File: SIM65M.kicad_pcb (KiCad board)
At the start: 4 copper layers, 40 x 40 mm, 25 parts, among them J1 Conn_01x11_Pin, J2 U.FL-R-SMT_10_, Q1 AO3400A, Q2 DTC143ZUAT106, Q3 DTC143ZUAT106, U1 SIM65M_C7495025, U2 BWGNSCNX25-25W4, U5 XC6206P282MR-G

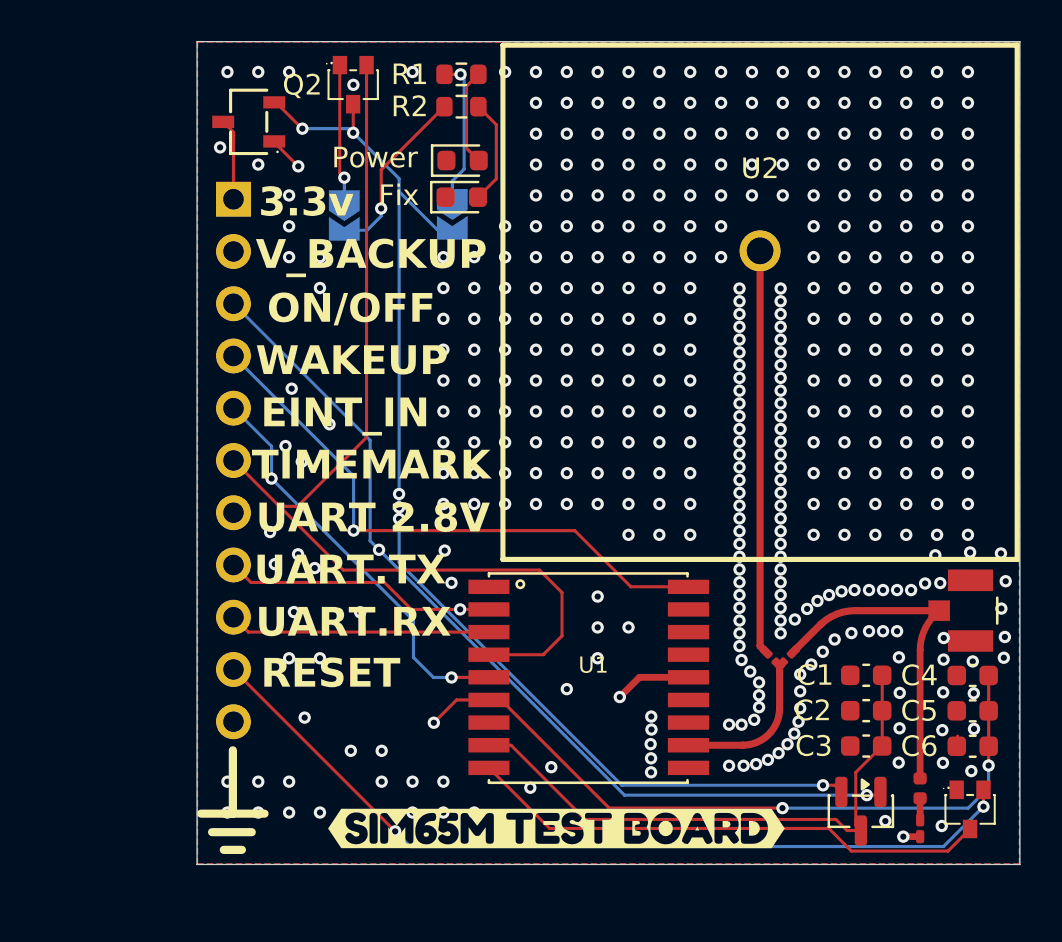
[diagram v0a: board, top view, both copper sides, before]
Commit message: carga
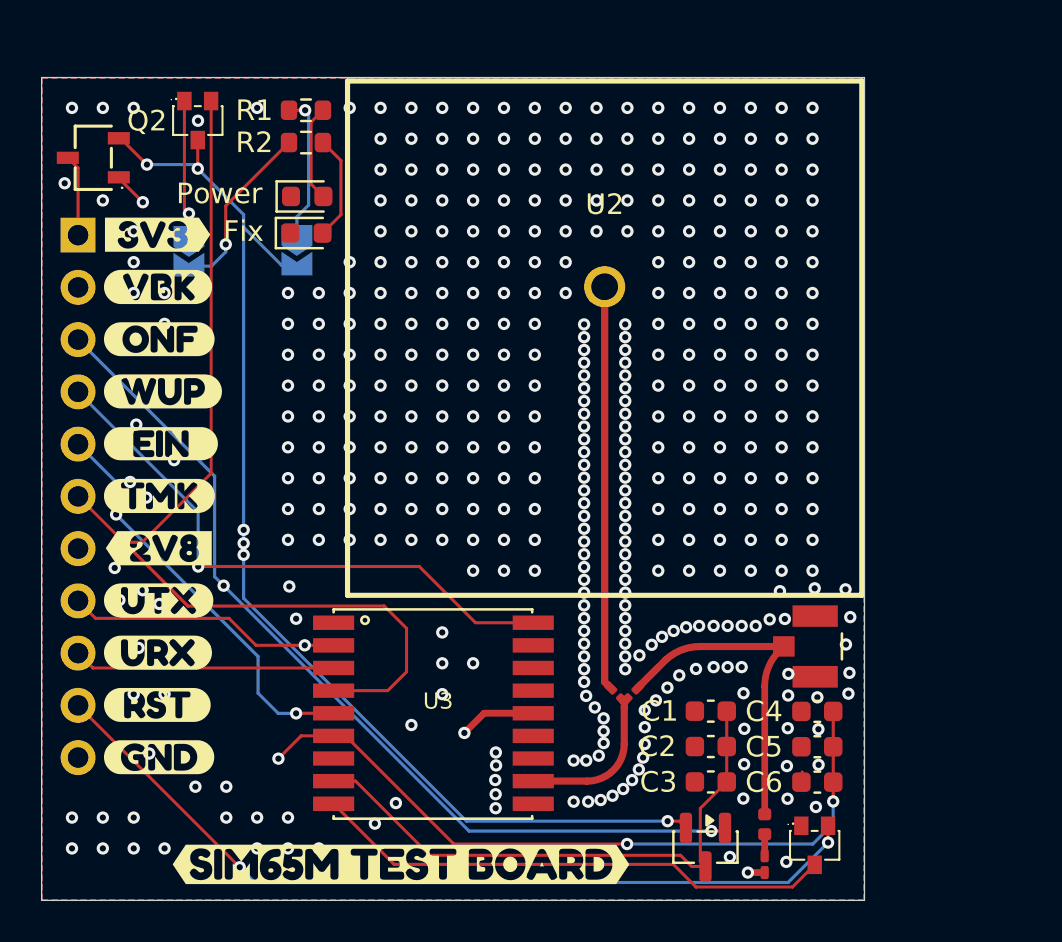
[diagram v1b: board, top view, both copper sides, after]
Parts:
- removed J2: U.FL-R-SMT_10_, Snapeda:U.FL-R-SMT_10_-foot
- removed U1: SIM65M_C7495025, Snapeda:SIM65M_foot
- added J3: U.FL-R-SMT_10_, Snapeda:U.FL-R-SMT_10_-foot, F.Cu at (221.4, 104.3)
- added U3: SIM65M_C7495025, Snapeda:SIM65M_foot, F.Cu at (203.1, 106.9)
- added kibuzzard-6A7951F5: G***, kibuzzard-6A7951F5, F.Cu at (189.7, 91.9)
- added kibuzzard-6A795201: G***, kibuzzard-6A795201, F.Cu at (189.5, 96.9)
- added kibuzzard-6A795219: G***, kibuzzard-6A795219, F.Cu at (189.5, 102.0)
- added kibuzzard-6A79521E: G***, kibuzzard-6A79521E, F.Cu at (189.4, 104.6)
- added kibuzzard-6A795229: G***, kibuzzard-6A795229, F.Cu at (189.5, 109.6)
- added kibuzzard-6A79523C: G***, kibuzzard-6A79523C, F.Cu at (189.4, 86.8)
- added kibuzzard-6A795244: G***, kibuzzard-6A795244, F.Cu at (189.5, 89.3)
- added kibuzzard-6A79525C: G***, kibuzzard-6A79525C, F.Cu at (189.6, 94.4)
- added kibuzzard-6A795279: G***, kibuzzard-6A795279, F.Cu at (189.4, 107.1)
- added kibuzzard-6A7952C3: G***, kibuzzard-6A7952C3, F.Cu at (189.5, 99.5)
- added kibuzzard-6A795305: G***, kibuzzard-6A795305, F.Cu at (189.4, 84.2)
- moved C1 7.75 mm to (216.3, 107.4)
- moved C2 7.75 mm to (216.3, 109.1)
- moved C3 7.75 mm to (216.3, 110.8)
- moved C6 7.75 mm to (221.5, 110.9)
- moved D1 7.75 mm to (196.7, 82.4)
- moved J1 7.75 mm to (185.5, 84.3)
- moved JP1 7.75 mm to (196.2, 85.0)
- moved JP2 7.75 mm to (190.9, 85.0)
- moved Q1 7.75 mm to (216.0, 114.0)
- moved R2 7.75 mm to (196.6, 79.8)
- moved kibuzzard-6A279BE5 7.75 mm to (201.2, 114.9)
- moved C4 7.75 mm to (221.5, 107.4)
- moved C5 7.75 mm to (221.5, 109.1)
- moved Q3 7.75 mm to (221.4, 113.9)
- moved R1 7.75 mm to (196.6, 78.2)
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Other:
- board text removed: "3.3v"
- board text removed: "EINT_IN"
- board text removed: "ON/OFF"
- board text removed: "RESET"
- board text removed: "TIMEMARK"
- board text removed: "UART 2.8V"
- board text removed: "UART.RX"
- board text removed: "UART.TX"
- board text removed: "V_BACKUP"
- board text removed: "WAKEUP"
